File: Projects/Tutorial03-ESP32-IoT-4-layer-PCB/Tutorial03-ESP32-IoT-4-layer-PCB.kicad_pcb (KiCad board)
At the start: 4 copper layers, 88 x 55.8 mm, 92 parts, among them J1 SS-52400-002, J2 B2B-PH-SM4-TB, J3 GSD090012SEU, J4 Conn_01x04_Pin, J5 Conn_01x05_Pin, Q1 TEMT6000X01, Q2 BC817, Q3 BC817, U1 MCP73871, U2 MAX4466EXK, U3 ESP32-C3-WROOM-02-H4, U4 CP2102N-Axx-xQFN20, U5 USBLC6-2SC6, U6 W25Q32JVSSIQ, U7 BME280

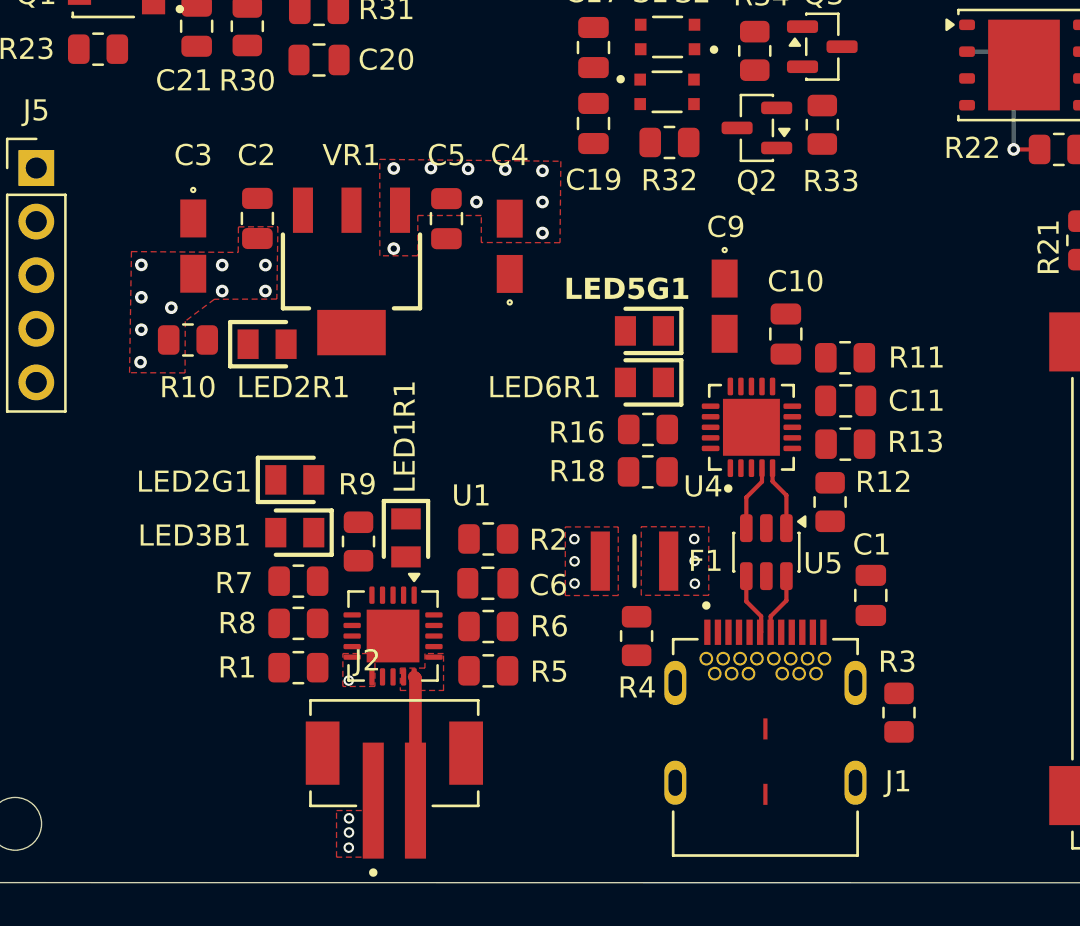
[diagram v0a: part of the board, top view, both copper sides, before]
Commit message: 20260718
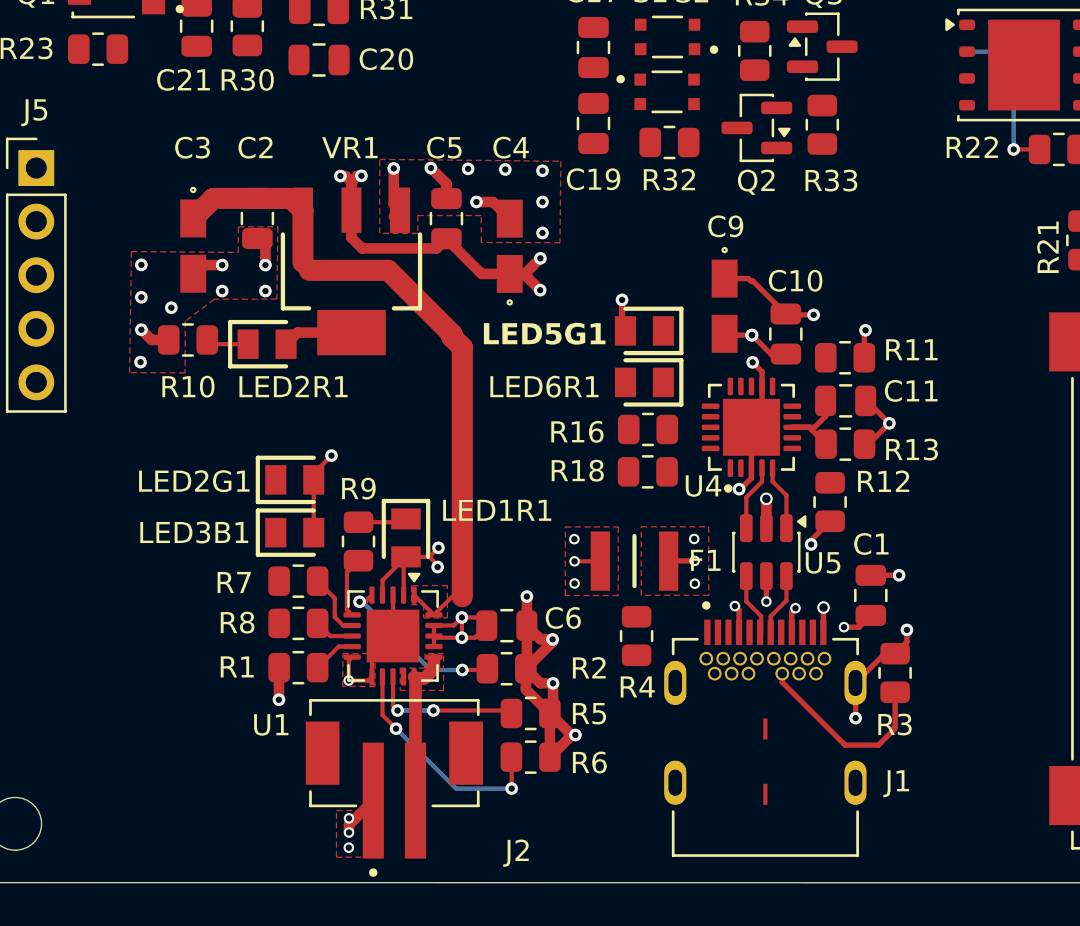
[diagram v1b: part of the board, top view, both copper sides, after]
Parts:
- moved R6 6.51 mm to (121.4, 112.4)
- moved R2 6.21 mm to (120.3, 108.2)
- moved R5 2.85 mm to (121.4, 110.4)
- moved C6 2.20 mm to (120.3, 106.2)
- moved R3 1.89 mm to (138.7, 108.5)
- turned LED3B1 to 0 degrees
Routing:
- net GND: track 5.87 -> 68.6 mm, vias 22 -> 35
- net +5V: track 0.00 -> 32.0 mm
- net +3.3V: track 5.83 -> 30.6 mm, vias 0 -> 8
- net /+5V_USB: track 0.00 -> 19.3 mm, vias 3 -> 8
- net Net-(U1-PROG3): track 0.00 -> 10.9 mm, vias 0 -> 2
- net Net-(J1-CC2): track 0.00 -> 9.04 mm
- net Net-(U1-THERM): track 0.00 -> 8.14 mm, vias 0 -> 2
- net /VBUS: track 0.00 -> 7.95 mm, vias 3 -> 8
- net Net-(U1-PROG1): track 0.00 -> 7.14 mm, vias 0 -> 2
- net Net-(U4-VBUS): track 0.00 -> 4.45 mm
- net /POWER_CHARGING_GOOD: track 0.00 -> 3.03 mm
- net /CHARGING: track 0.00 -> 2.90 mm
- net Net-(LED1R1-K): track 0.00 -> 2.32 mm
- net Net-(U1-~{TE}): track 0.00 -> 2.05 mm
- net Net-(LED2R1-K): track 0.00 -> 2.02 mm
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- added copper zone on F.Cu, net +5V

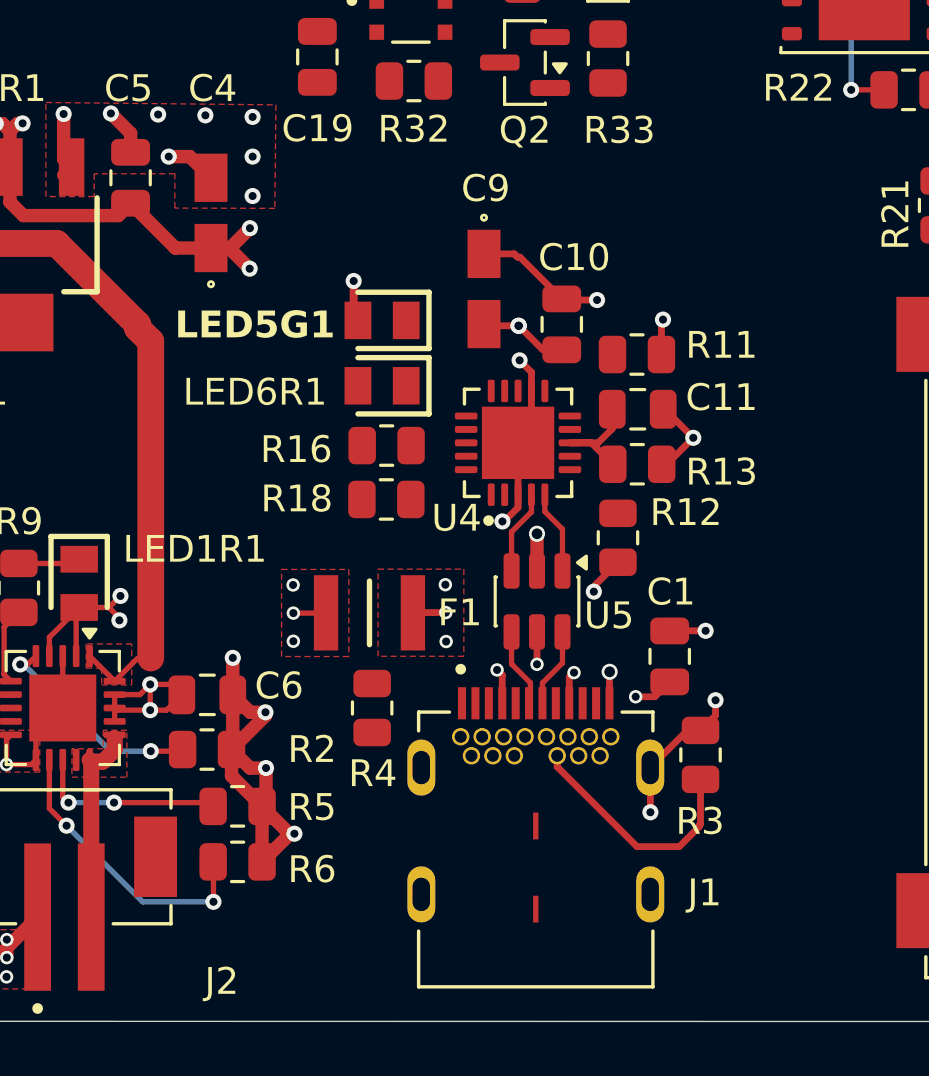
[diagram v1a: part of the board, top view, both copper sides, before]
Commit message: 20260718
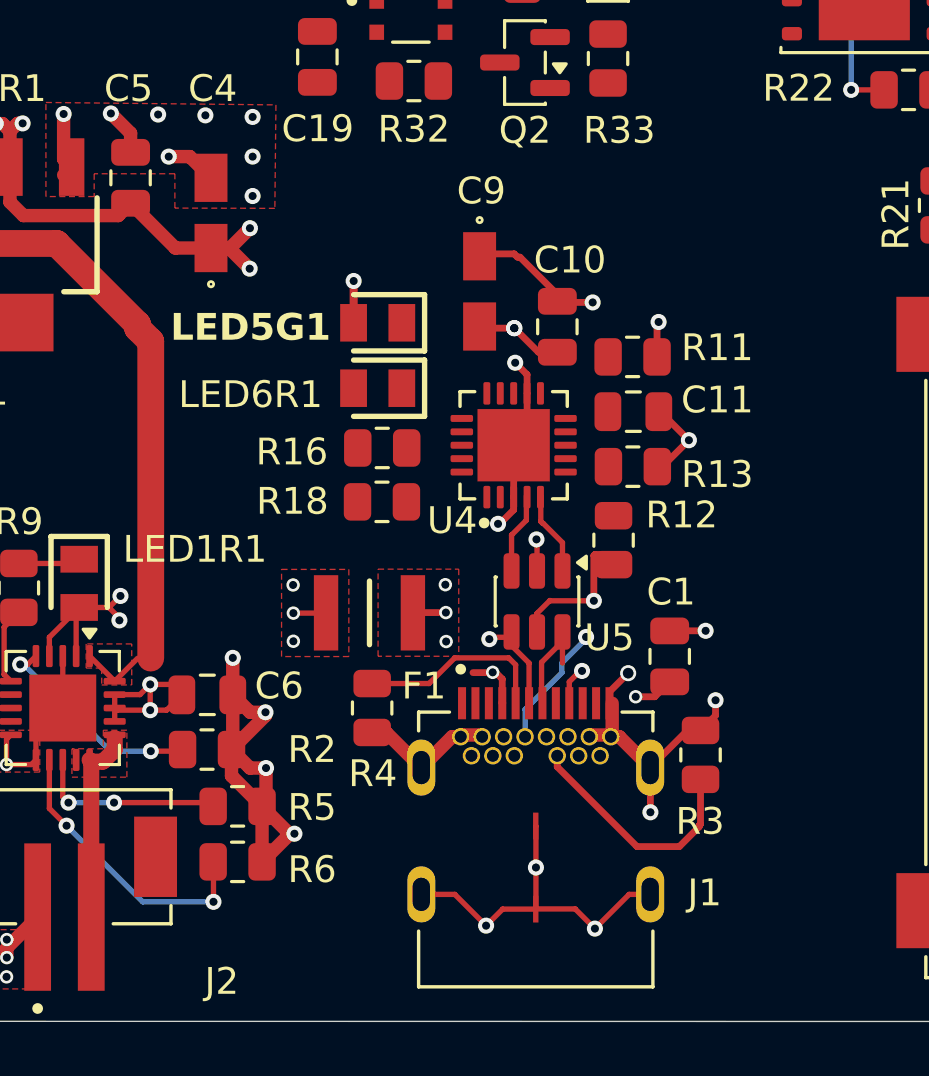
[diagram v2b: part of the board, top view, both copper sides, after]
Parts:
- moved C10 0.19 mm to (133.4, 92.5)
- moved C9 0.19 mm to (130.5, 91.2)
- moved R12 0.19 mm to (135.5, 100.4)
- moved R13 0.19 mm to (136.2, 97.7)
- moved R16 0.19 mm to (126.8, 97.0)
- moved R18 0.19 mm to (126.8, 99.0)
- moved R11 0.19 mm to (136.2, 93.6)
- moved U4 0.19 mm to (131.7, 96.9)
- moved LED5G1 0.19 mm to (126.7, 92.3)
- moved LED6R1 0.19 mm to (126.7, 94.8)
- moved C11 0.19 mm to (136.2, 95.6)
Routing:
- net GND: track 68.6 -> 91.1 mm, vias 35 -> 38
- net Net-(J1-CC1): track 0.00 -> 7.29 mm
- net /USB_DN: track 2.97 -> 8.89 mm, vias 0 -> 1
- net /USB_DP: track 3.00 -> 8.40 mm, vias 0 -> 1
- net Net-(U4-VBUS): track 4.45 -> 0.00 mm
- net /VBUS: track 7.95 -> 12.3 mm, vias 8 -> 7

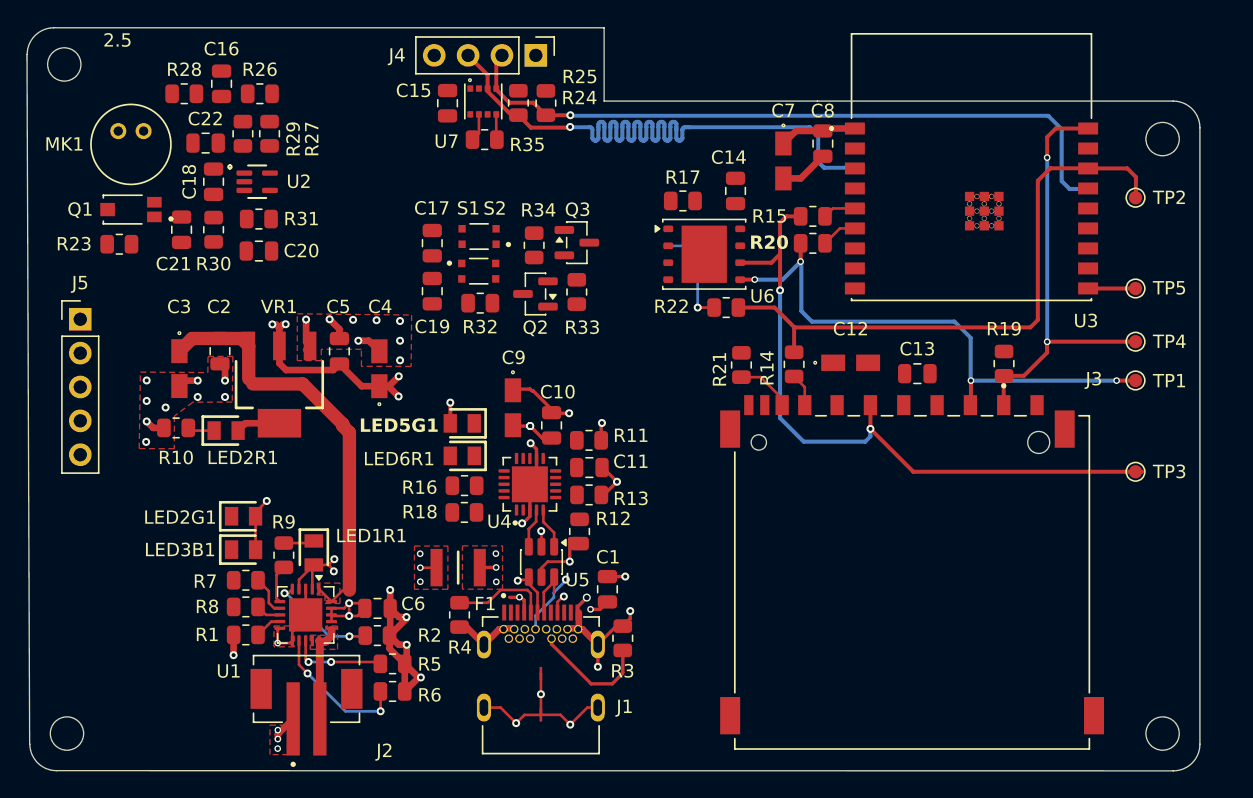
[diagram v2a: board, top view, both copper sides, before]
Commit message: 20260726
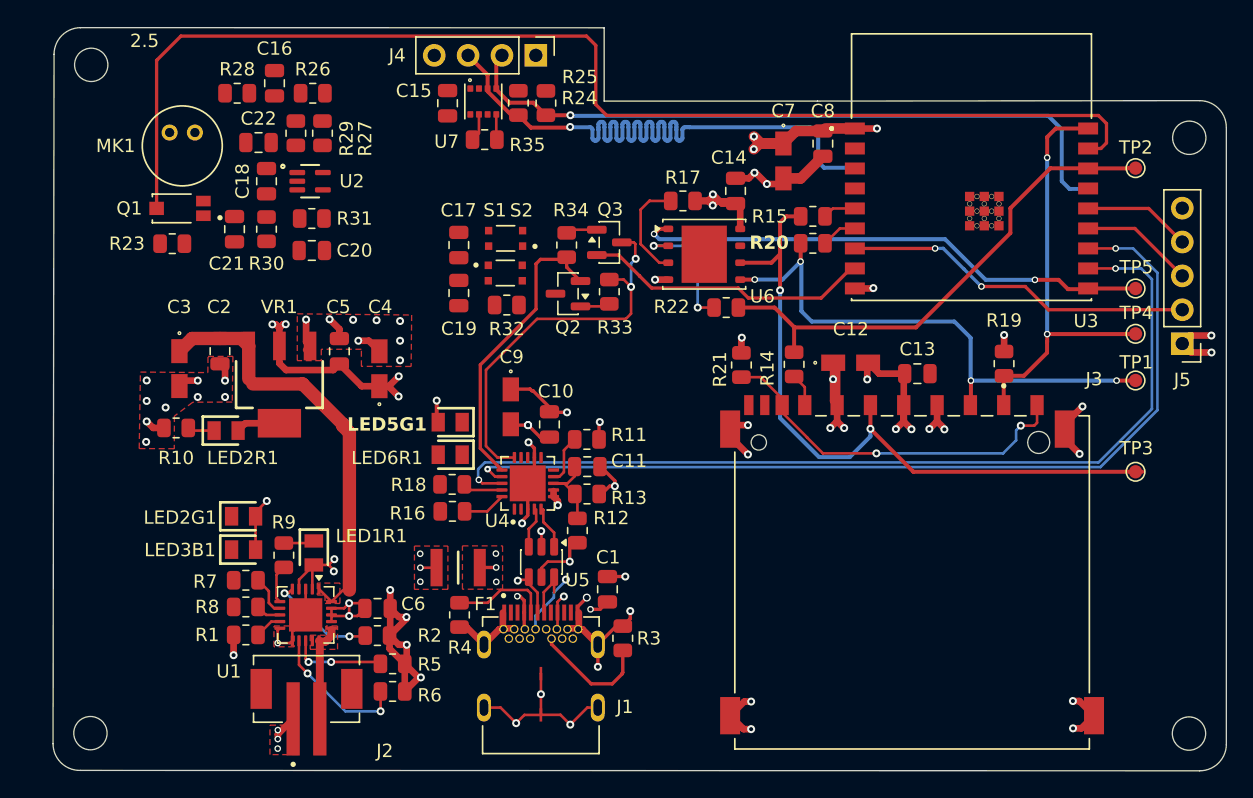
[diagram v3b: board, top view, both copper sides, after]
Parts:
- moved J5 82.7 mm to (180.7, 86.3), turned to 180 degrees
- moved C16 3.97 mm to (112.6, 66.8)
- moved C18 3.97 mm to (112.0, 74.2)
- moved C20 3.97 mm to (115.4, 79.4)
- moved C21 3.97 mm to (109.6, 77.8)
- moved C22 3.97 mm to (111.4, 71.3)
- moved R23 3.97 mm to (104.9, 78.8)
- moved R26 3.97 mm to (115.4, 67.6)
- moved R27 3.97 mm to (116.2, 70.6)
- moved R28 3.97 mm to (109.8, 67.6)
- moved R29 3.97 mm to (114.2, 70.6)
- moved R30 3.97 mm to (112.0, 77.8)
- moved R31 3.97 mm to (115.4, 77.0)
- moved U2 3.97 mm to (115.2, 74.2)
- moved MK1 3.85 mm to (105.7, 71.5)
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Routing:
- net /ESP-32-C3-02/PHOTO_C: track 0.00 -> 91.5 mm
- net /ESP-32-C3-02/TX_RX: track 0.00 -> 70.0 mm, vias 0 -> 2
- net /ESP-32-C3-02/RX_TX: track 0.00 -> 69.7 mm, vias 0 -> 2
- net GND: track 91.1 -> 129.1 mm, vias 38 -> 56
- net /ESP-32-C3-02/CS: track 3.56 -> 39.1 mm, vias 0 -> 2
- net +3.3V: track 30.6 -> 64.2 mm, vias 8 -> 20
- net /ESP-32-C3-02/DTR: track 0.00 -> 29.1 mm, vias 0 -> 2
- net /ESP-32-C3-02/GPIO8: track 0.00 -> 26.5 mm, vias 0 -> 2
- net Net-(J3-DAT1): track 4.22 -> 27.9 mm, vias 0 -> 2
- net /ESP-32-C3-02/RTS: track 0.00 -> 22.1 mm
- net /ESP-32-C3-02/BOOT: track 0.00 -> 21.6 mm
- net /ESP-32-C3-02/GPIO18: track 0.00 -> 8.54 mm
- net /ESP-32-C3-02/GPIO19: track 0.00 -> 8.11 mm
- net Net-(U6-~{HOLD}/~{RESET}(IO3)): track 0.00 -> 7.78 mm
- net /ESP-32-C3-02/MISO_DO: track 45.2 -> 38.3 mm
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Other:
- outline, holes or cut-outs redrawn

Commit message: 20260801
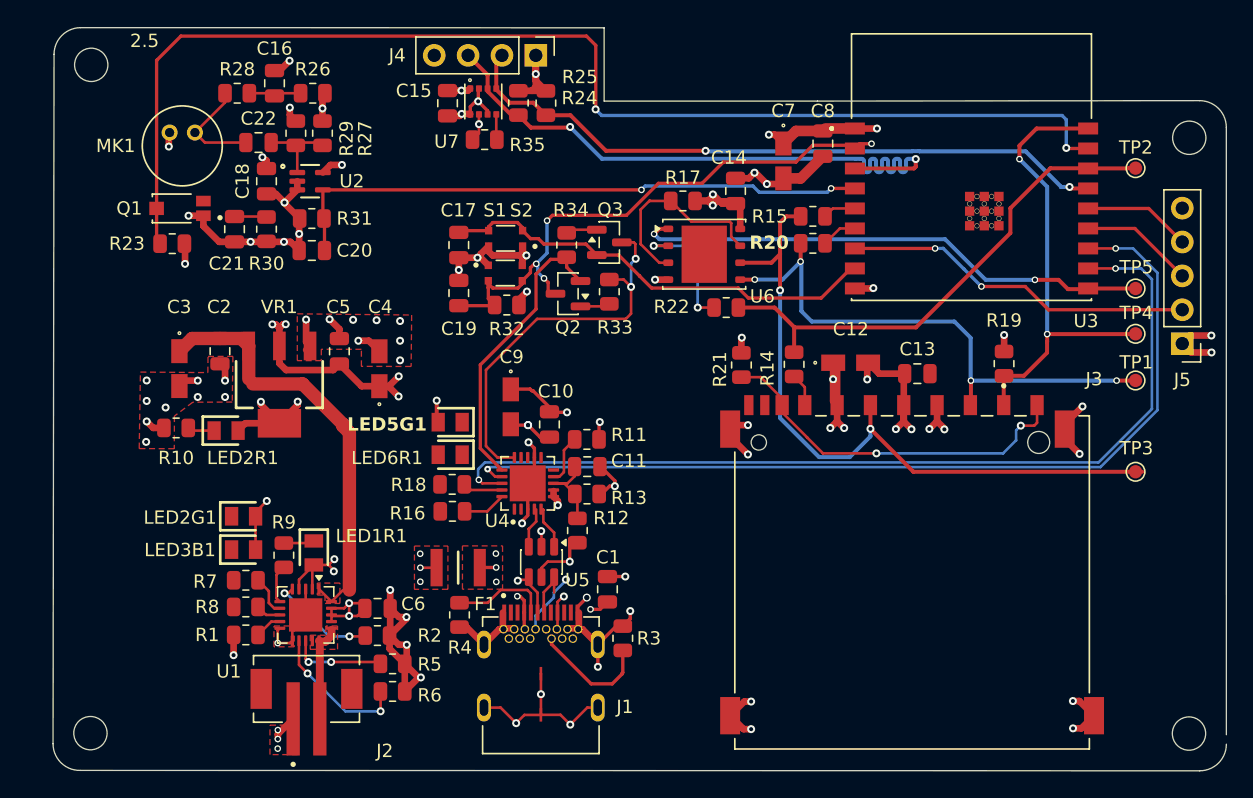
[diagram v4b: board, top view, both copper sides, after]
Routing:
- net /ESP-32-C3-02/MIC_OUT: track 0.00 -> 44.9 mm, vias 0 -> 2
- net /ESP-32-C3-02/EN: track 0.00 -> 43.9 mm, vias 0 -> 4
- net GND: track 129.1 -> 163.1 mm, vias 56 -> 69
- net +3.3V: track 64.2 -> 86.6 mm, vias 20 -> 29
- net /ESP-32-C3-02/BOOT: track 21.6 -> 33.6 mm
- net Net-(C22-Pad1): track 0.00 -> 8.02 mm
- net Net-(U6-~{HOLD}/~{RESET}(IO3)): track 7.78 -> 15.0 mm
- net Net-(U2-IN+): track 0.00 -> 6.02 mm
- net Net-(C16-Pad2): track 0.00 -> 3.84 mm
- net /ESP-32-C3-02/SDA: track 53.1 -> 49.7 mm, vias 1 -> 2
- net /ESP-32-C3-02/CS_SD: track 31.9 -> 34.4 mm
- net Net-(C21-Pad1): track 0.00 -> 2.42 mm
- net /ESP-32-C3-02/SCL: track 52.6 -> 50.3 mm, vias 1 -> 2
- net /ESP-32-C3-02/PHOTO_C: track 91.5 -> 92.1 mm, vias 0 -> 2
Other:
- outline, holes or cut-outs redrawn

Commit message: 20260808
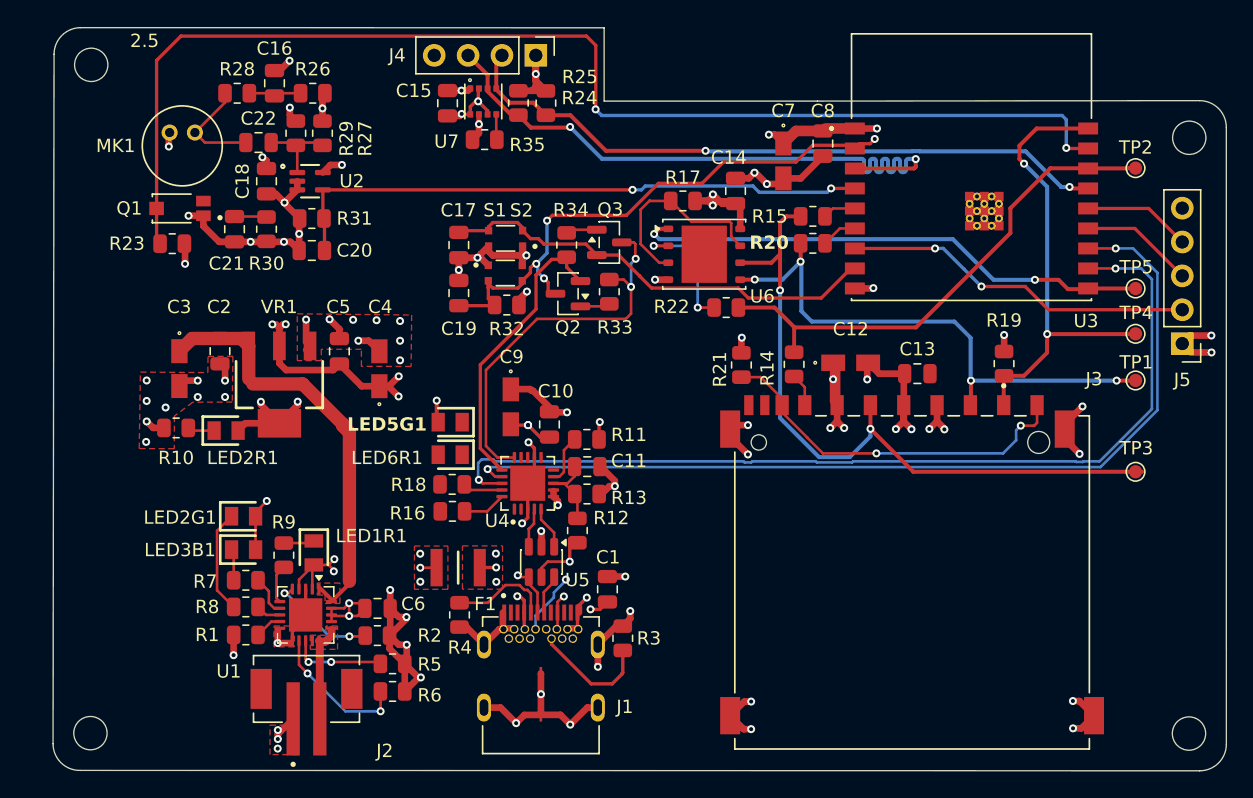
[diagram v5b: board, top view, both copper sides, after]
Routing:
- net GND: track 163.1 -> 173.4 mm
- net Net-(LED2G1-K): track 0.00 -> 7.77 mm
- net Net-(LED3B1-K): track 0.00 -> 2.37 mm
- net /USB_DN: track 8.89 -> 7.73 mm
- net /USB_DP: track 8.40 -> 9.02 mm
- net /ESP-32-C3-02/TX_RX: track 70.0 -> 70.5 mm
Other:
- outline, holes or cut-outs redrawn
